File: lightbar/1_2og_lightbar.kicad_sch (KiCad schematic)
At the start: 35 parts, among them J1 Conn_01x03

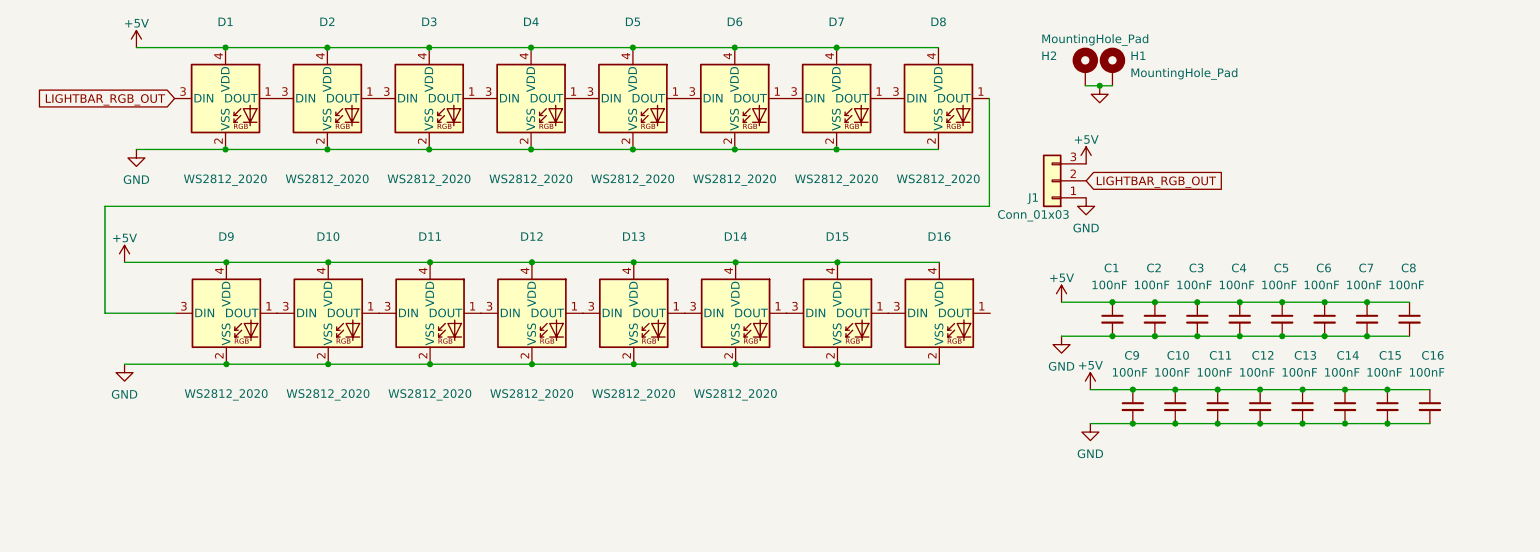
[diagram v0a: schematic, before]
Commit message: idk
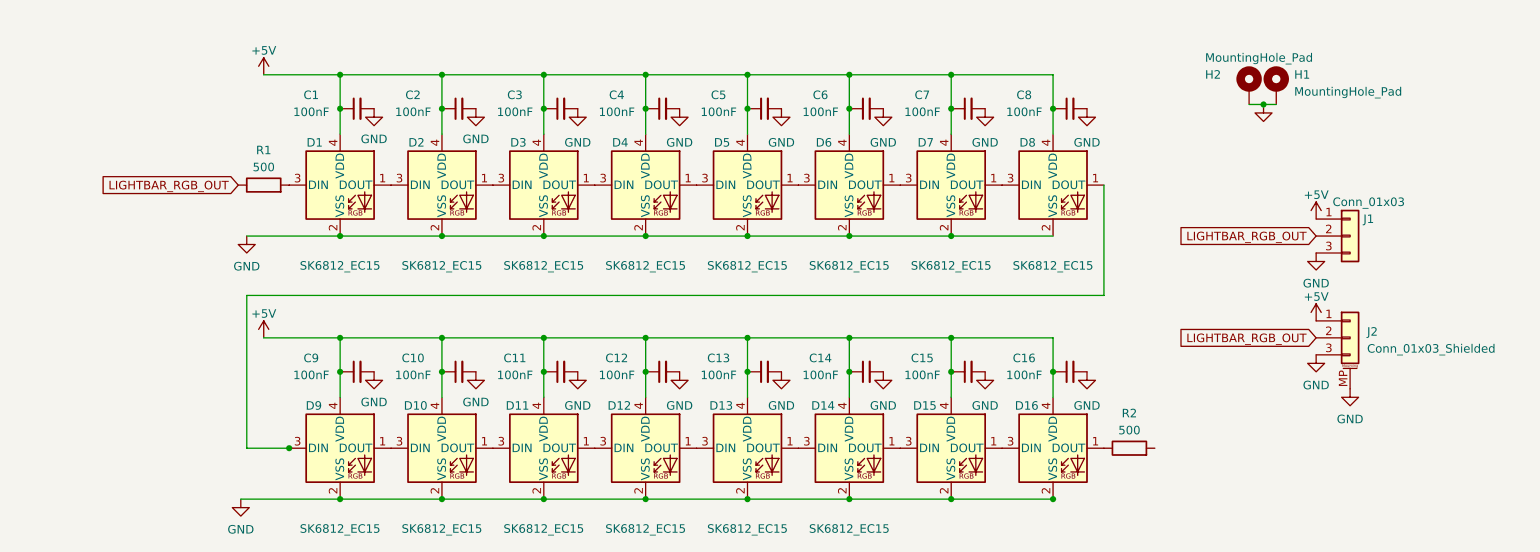
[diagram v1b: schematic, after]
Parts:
- added J2: Conn_01x03_Shielded, Connector_Molex:Molex_Pico-EZmate_78171-0003_1x03-1MP_P1.20mm_Vertical, symbol Connector_Generic_MountingPin:Conn_01x03_MountingPin
- added R1, R2: 500, Resistor_SMD:R_0805_2012Metric, symbol Device:R
- C1, C10, C11, C12, C13, C14, C15, C16, C2, C3, C4, C5, C6, C7, C8, C9: LCSC C1525 -> (none)
- D1, D10, D11, D12, D13, D14, D15, D16, D2, D3, D4, D5, D6, D7, D8, D9: value WS2812_2020 -> SK6812_EC15; footprint marbastlib-various:LED_WS2812_2020 -> LED_SMD:LED_SK6812_EC15_1.5x1.5mm; symbol marbastlib-various:WS2812_2020 -> LED:SK6805
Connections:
- net +5V: now also J1.1 (Pin_1), J2.1 (Pin_1); no longer J1.3 (Pin_3)
- net GND: now also J1.3 (Pin_3), J2.3 (Pin_3), J2.MP (MountPin); no longer J1.1 (Pin_1)
- net LIGHTBAR_RGB_OUT: now also J2.2 (Pin_2), R1.1; no longer D1.3 (DIN)
- net at D16.1 (DOUT): now also R2.1
- new net: D1.3 (DIN), R1.2
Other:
- moved on the sheet: D1, D10, D11, D12, D13, D14, D15, D16, D2, D3, D4, D5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
